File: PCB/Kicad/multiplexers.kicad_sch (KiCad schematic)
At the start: 4 parts

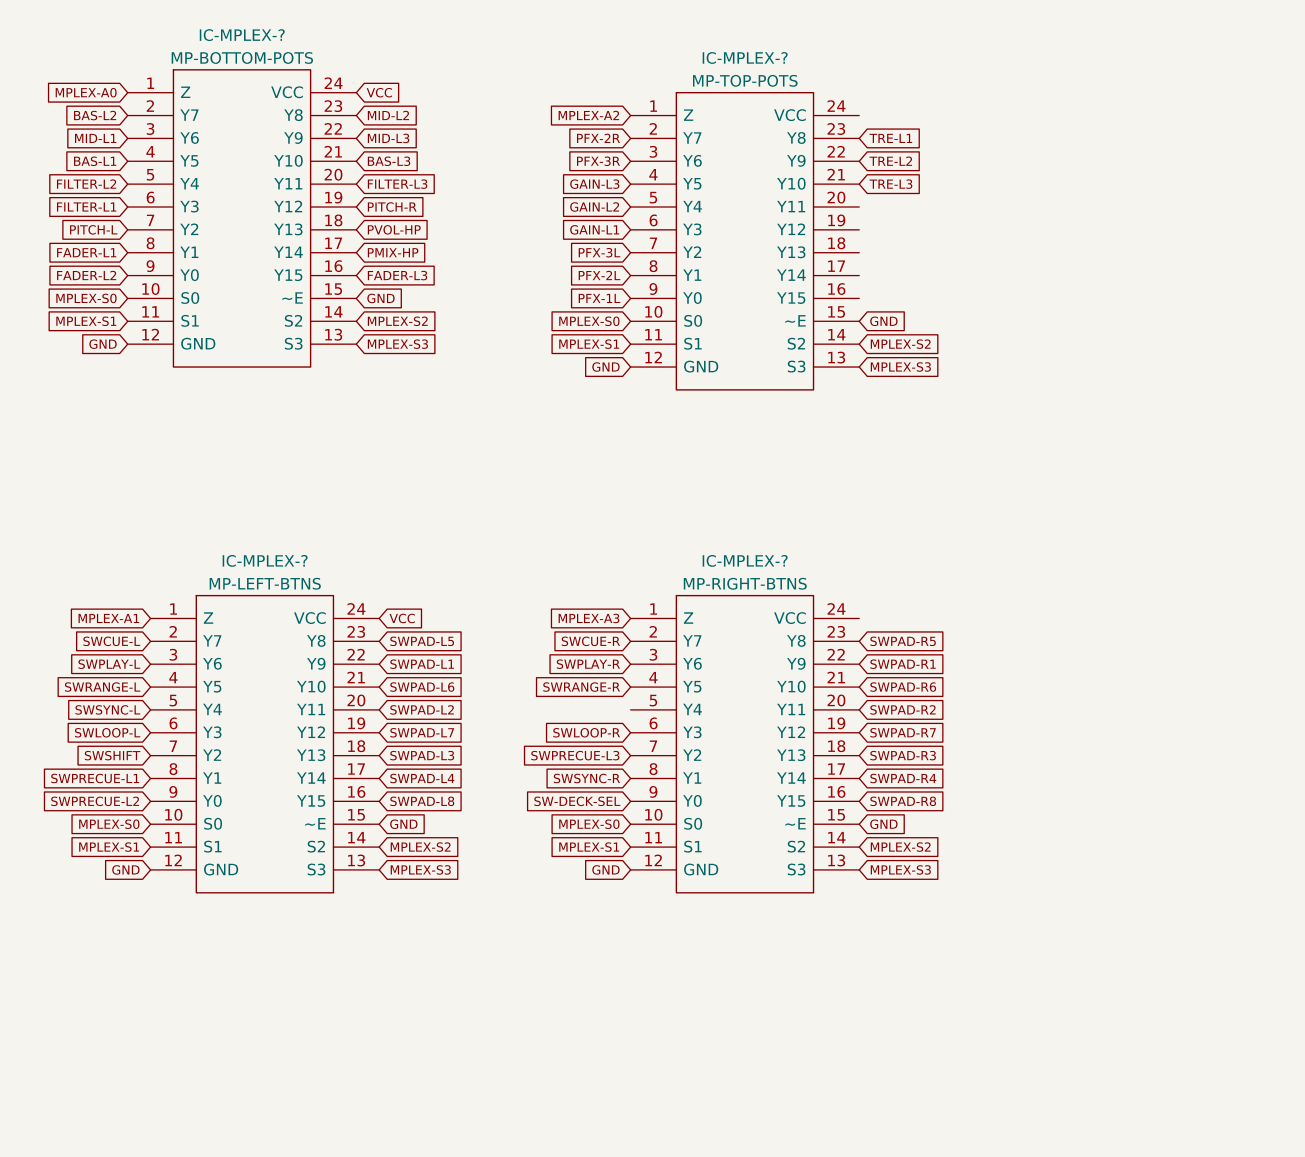
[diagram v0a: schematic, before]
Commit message: SCHEMATIC FINISHED
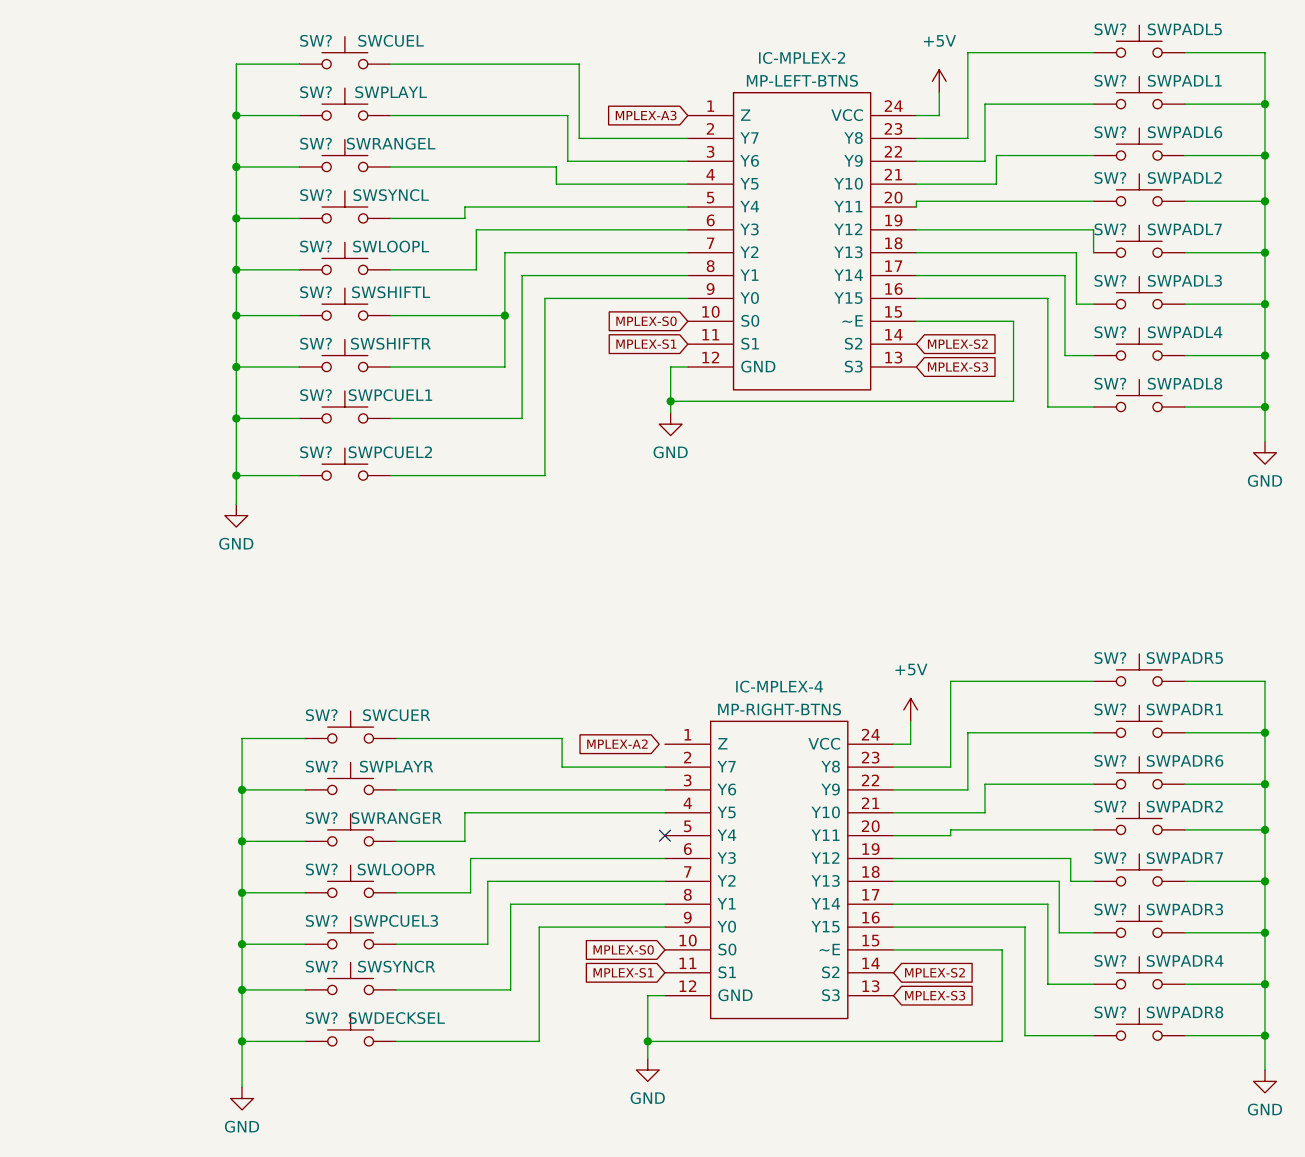
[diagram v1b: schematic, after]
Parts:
- removed IC-MPLEX-?: MP-BOTTOM-POTS, Library:SOIC-24W_7.5x15.4mm_P1.27mm, symbol mixduino-mk2:74HC4067D,653
- removed IC-MPLEX-?: MP-TOP-POTS, Library:SOIC-24W_7.5x15.4mm_P1.27mm, symbol mixduino-mk2:74HC4067D,653
- added SW?: SWPADR7, Library:sw-pad, symbol mixduino-mk2:SW_Push
- added SW?: SWSYNCR, Library:SW_PUSH_6mm_H8mm, symbol mixduino-mk2:SW_Push
- added SW?: SWSHIFTR, Library:SW_PUSH_6mm_H8mm, symbol mixduino-mk2:SW_Push
- added SW?: SWLOOPR, Library:SW_PUSH_6mm_H8mm, symbol mixduino-mk2:SW_Push
- added SW?: SWPADR2, Library:sw-pad, symbol mixduino-mk2:SW_Push
- added SW?: SWPLAYL, Library:SW_PUSH_6mm_H8mm, symbol mixduino-mk2:SW_Push
- added SW?: SWPADR8, Library:sw-pad, symbol mixduino-mk2:SW_Push
- added SW?: SWPADR1, Library:sw-pad, symbol mixduino-mk2:SW_Push
- added SW?: SWPCUEL3, Library:SW_PUSH_6mm_H8mm, symbol mixduino-mk2:SW_Push
- added SW?: SWPCUEL2, Library:SW_PUSH_6mm_H8mm, symbol mixduino-mk2:SW_Push
- added SW?: SWPADR3, Library:sw-pad, symbol mixduino-mk2:SW_Push
- added SW?: SWSHIFTL, Library:SW_PUSH_6mm_H8mm, symbol mixduino-mk2:SW_Push
- added SW?: SWPADL4, Library:sw-pad, symbol mixduino-mk2:SW_Push
- added SW?: SWPADR5, Library:sw-pad, symbol mixduino-mk2:SW_Push
- added SW?: SWPCUEL1, Library:SW_PUSH_6mm_H8mm, symbol mixduino-mk2:SW_Push
- added SW?: SWPADR4, Library:sw-pad, symbol mixduino-mk2:SW_Push
- added SW?: SWSYNCL, Library:SW_PUSH_6mm_H8mm, symbol mixduino-mk2:SW_Push
- added SW?: SWPADL7, Library:sw-pad, symbol mixduino-mk2:SW_Push
- added SW?: SWPADL5, Library:sw-pad, symbol mixduino-mk2:SW_Push
- added SW?: SWPADL3, Library:sw-pad, symbol mixduino-mk2:SW_Push
- added SW?: SWPADL1, Library:sw-pad, symbol mixduino-mk2:SW_Push
- added SW?: SWDECKSEL, Library:SW_PUSH_6mm_H8mm, symbol mixduino-mk2:SW_Push
- added SW?: SWPADL8, Library:sw-pad, symbol mixduino-mk2:SW_Push
- added SW?: SWPADL2, Library:sw-pad, symbol mixduino-mk2:SW_Push
- added SW?: SWRANGEL, Library:SW_PUSH_6mm_H8mm, symbol mixduino-mk2:SW_Push
- added SW?: SWLOOPL, Library:SW_PUSH_6mm_H8mm, symbol mixduino-mk2:SW_Push
- added SW?: SWRANGER, Library:SW_PUSH_6mm_H8mm, symbol mixduino-mk2:SW_Push
- added SW?: SWCUEL, Library:SW_PUSH_6mm_H8mm, symbol mixduino-mk2:SW_Push
- added SW?: SWPADL6, Library:sw-pad, symbol mixduino-mk2:SW_Push
- added SW?: SWPADR6, Library:sw-pad, symbol mixduino-mk2:SW_Push
- added SW?: SWPLAYR, Library:SW_PUSH_6mm_H8mm, symbol mixduino-mk2:SW_Push
- added SW?: SWCUER, Library:SW_PUSH_6mm_H8mm, symbol mixduino-mk2:SW_Push
- gave numbers to parts that had none: 2
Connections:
- net MPLEX-A1 is gone; now on net MPLEX-A3: IC-MPLEX-2.1 (Z)
- net VCC is gone; now on net +5V: IC-MPLEX-2.24 (VCC)
- net GND: now also SW?.1, SW?.1, SW?.1, SW?.1, SW?.1, SW?.1, SW?.1, SW?.1, SW?.1, SW?.1, SW?.1, SW?.1, SW?.1, SW?.1, SW?.1, SW?.1, SW?.2, SW?.2, SW?.2, SW?.2, SW?.2, SW?.2, SW?.2, SW?.2, SW?.2, SW?.2, SW?.2, SW?.2, SW?.2, SW?.2, SW?.2, SW?.2
- net MPLEX-A3: no longer IC-MPLEX-4.1 (Z)
- net +5V: now reaches IC-MPLEX-4.24 (VCC)
- net SW-DECK-SEL: no longer names the net of IC-MPLEX-4.9 (Y0)
- net SW-DECK-SEL: now also SW?.2
- net SWCUE-L: no longer names the net of IC-MPLEX-2.2 (Y7)
- net SWCUE-L: now also SW?.2
- net SWCUE-R: no longer names the net of IC-MPLEX-4.2 (Y7)
- net SWCUE-R: now also SW?.2
- net SWLOOP-L: no longer names the net of IC-MPLEX-2.6 (Y3)
- net SWLOOP-L: now also SW?.2
- net SWLOOP-R: no longer names the net of IC-MPLEX-4.6 (Y3)
- net SWLOOP-R: now also SW?.2
- net SWPAD-L1: no longer names the net of IC-MPLEX-2.22 (Y9)
- net SWPAD-L1: now also SW?.1
- net SWPAD-L2: no longer names the net of IC-MPLEX-2.20 (Y11)
- net SWPAD-L2: now also SW?.1
- net SWPAD-L3: no longer names the net of IC-MPLEX-2.18 (Y13)
- net SWPAD-L3: now also SW?.1
- net SWPAD-L4: no longer names the net of IC-MPLEX-2.17 (Y14)
- net SWPAD-L4: now also SW?.1
- net SWPAD-L5: no longer names the net of IC-MPLEX-2.23 (Y8)
- net SWPAD-L5: now also SW?.1
- net SWPAD-L6: no longer names the net of IC-MPLEX-2.21 (Y10)
- net SWPAD-L6: now also SW?.1
- net SWPAD-L7: no longer names the net of IC-MPLEX-2.19 (Y12)
- net SWPAD-L7: now also SW?.1
- net SWPAD-L8: no longer names the net of IC-MPLEX-2.16 (Y15)
- net SWPAD-L8: now also SW?.1
- net SWPAD-R1: no longer names the net of IC-MPLEX-4.22 (Y9)
- net SWPAD-R1: now also SW?.1
- net SWPAD-R2: no longer names the net of IC-MPLEX-4.20 (Y11)
- net SWPAD-R2: now also SW?.1
- net SWPAD-R3: no longer names the net of IC-MPLEX-4.18 (Y13)
- net SWPAD-R3: now also SW?.1
- net SWPAD-R4: no longer names the net of IC-MPLEX-4.17 (Y14)
- net SWPAD-R4: now also SW?.1
- net SWPAD-R5: no longer names the net of IC-MPLEX-4.23 (Y8)
- net SWPAD-R5: now also SW?.1
- net SWPAD-R6: no longer names the net of IC-MPLEX-4.21 (Y10)
- net SWPAD-R6: now also SW?.1
- net SWPAD-R7: no longer names the net of IC-MPLEX-4.19 (Y12)
- net SWPAD-R7: now also SW?.1
- net SWPAD-R8: no longer names the net of IC-MPLEX-4.16 (Y15)
- net SWPAD-R8: now also SW?.1
- net SWPLAY-L: no longer names the net of IC-MPLEX-2.3 (Y6)
- net SWPLAY-L: now also SW?.2
- net SWPLAY-R: no longer names the net of IC-MPLEX-4.3 (Y6)
- net SWPLAY-R: now also SW?.2
- net SWPRECUE-L1: no longer names the net of IC-MPLEX-2.8 (Y1)
- net SWPRECUE-L1: now also SW?.2
- net SWPRECUE-L2: no longer names the net of IC-MPLEX-2.9 (Y0)
- net SWPRECUE-L2: now also SW?.2
- net SWPRECUE-L3: no longer names the net of IC-MPLEX-4.7 (Y2)
- net SWPRECUE-L3: now also SW?.2
- net SWRANGE-L: no longer names the net of IC-MPLEX-2.4 (Y5)
- net SWRANGE-L: now also SW?.2
- net SWRANGE-R: no longer names the net of IC-MPLEX-4.4 (Y5)
- net SWRANGE-R: now also SW?.2
- net SWSHIFT: no longer names the net of IC-MPLEX-2.7 (Y2)
- net SWSHIFT: now also SW?.2, SW?.2
- net SWSYNC-L: no longer names the net of IC-MPLEX-2.5 (Y4)
- net SWSYNC-L: now also SW?.2
- net SWSYNC-R: no longer names the net of IC-MPLEX-4.8 (Y1)
- net SWSYNC-R: now also SW?.2
- no-connect marks 0 -> 1
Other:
- moved on the sheet: IC-MPLEX-2, IC-MPLEX-4
